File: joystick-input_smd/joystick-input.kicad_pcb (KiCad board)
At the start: 2 copper layers, 53.3 x 35.1 mm, 22 parts, among them J1 Conn_02x18_Odd_Even, J2 Conn_02x14_Odd_Even

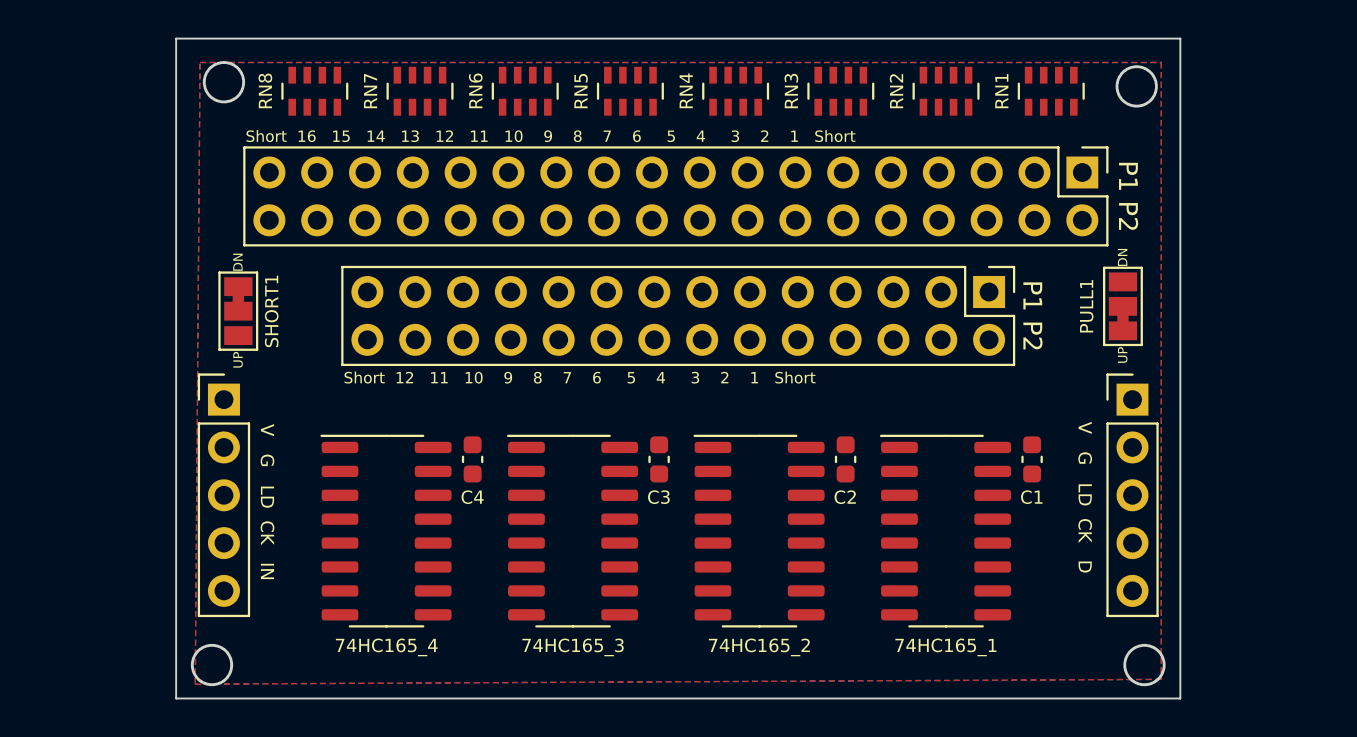
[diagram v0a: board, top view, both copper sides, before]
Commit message: 조이스틱 입력보드 smd 버전 1차 완성
Signed-off-by: Ju, Gyeong-min <jcmh74@gmail.com>
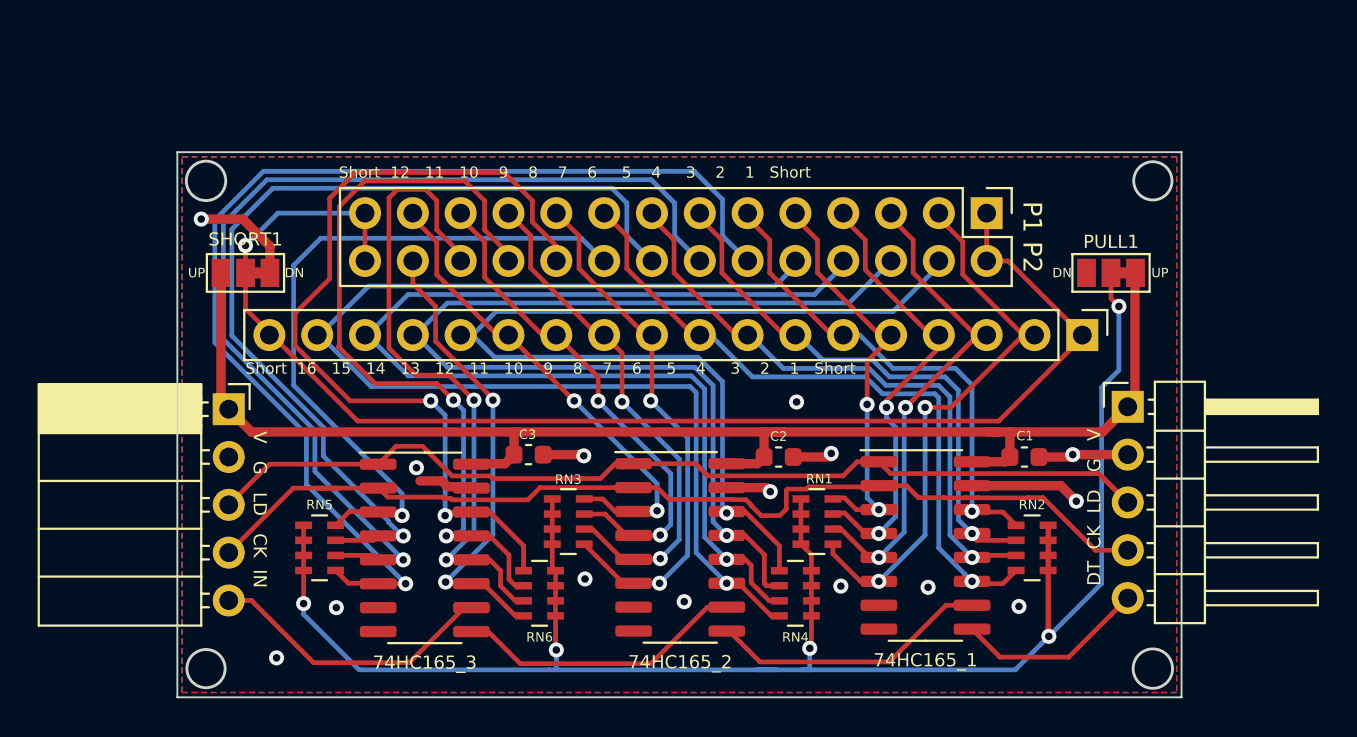
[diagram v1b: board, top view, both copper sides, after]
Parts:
- removed 74HC165_4: 74HC165, Package_SO:SOIC-16_3.9x9.9mm_P1.27mm
- removed C4: C, Capacitor_SMD:C_0603_1608Metric
- removed RN7, RN8: R_Pack04, Resistor_SMD:R_Array_Concave_4x0603
- IN1: footprint Connector_PinHeader_2.54mm:PinHeader_1x05_P2.54mm_Vertical -> Connector_PinSocket_2.54mm:PinSocket_1x05_P2.54mm_Horizontal
- J1: value Conn_02x18_Odd_Even -> Conn_01x18; footprint Connector_PinHeader_2.54mm:PinHeader_2x18_P2.54mm_Vertical -> Connector_PinHeader_2.54mm:PinHeader_1x18_P2.54mm_Vertical
- OUT1: footprint Connector_PinHeader_2.54mm:PinHeader_1x05_P2.54mm_Vertical -> Connector_PinHeader_2.54mm:PinHeader_1x05_P2.54mm_Horizontal
- moved RN5 29.3 mm to (119.4, 89.3), turned to 0 degrees
- moved RN3 27.1 mm to (132.6, 87.9), turned to 0 degrees
- moved RN4 26.9 mm to (144.7, 91.7), turned to 180 degrees
- moved RN6 26.7 mm to (131.1, 91.7), turned to 180 degrees
- moved RN1 26.0 mm to (145.8, 87.9), turned to 0 degrees
- moved RN2 24.7 mm to (157.2, 89.3), turned to 180 degrees
- moved J1 8.64 mm to (159.9, 78.0)
- moved 74HC165_3 7.92 mm to (125.0, 89.3)
- moved C3 6.94 mm to (130.5, 84.3), turned to 0 degrees
- moved 74HC165_2 4.30 mm to (138.5, 89.3)
- moved J2 4.19 mm to (154.8, 71.5)
- moved C2 3.56 mm to (143.8, 84.5), turned to 0 degrees
- moved SHORT1 2.07 mm to (115.4, 74.7), turned to 180 degrees
- moved PULL1 1.89 mm to (161.4, 74.7), turned to 180 degrees
- moved 74HC165_1 1.33 mm to (151.6, 89.2)
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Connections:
- 74HC165_2 pad 11: /C_P1_EX3 -> /C_P2_RIGHT
- 74HC165_2 pad 12: /C_P1_EX2 -> /C_P2_LEFT
- 74HC165_2 pad 13: /C_P1_EX1 -> /C_P2_DOWN
- 74HC165_2 pad 14: /C_P1_HK -> /C_P2_UP
- 74HC165_3 pad 10: /Q7_3 -> /D_IN
- 74HC165_3 pad 11: /C_P2_B -> /C_P2_R
- 74HC165_3 pad 12: /C_P2_A -> /C_P2_L
- 74HC165_3 pad 13: /C_P2_SELECT -> /C_P2_Y
- 74HC165_3 pad 14: /C_P2_START -> /C_P2_X
- 74HC165_3 pad 3: /C_P2_RIGHT -> /C_P2_B
- 74HC165_3 pad 4: /C_P2_LEFT -> /C_P2_A
- 74HC165_3 pad 5: /C_P2_DOWN -> /C_P2_SELECT
- 74HC165_3 pad 6: /C_P2_UP -> /C_P2_START
- J1 pad 10: /C_P2_RIGHT -> /C_P1_X
- J1 pad 11: /C_P1_START -> /C_P1_Y
- J1 pad 12: /C_P2_START -> /C_P1_L
- J1 pad 13: /C_P1_SELECT -> /C_P1_R
- J1 pad 14: /C_P2_SELECT -> /C_P2_UP
- J1 pad 15: /C_P1_A -> /C_P2_DOWN
- J1 pad 16: /C_P2_A -> /C_P2_LEFT
- J1 pad 17: /C_P1_B -> /C_P2_RIGHT
- J1 pad 18: /C_P2_B -> /C_SHORT
- J1 pad 2: /C_SHORT -> /C_P1_UP
- J1 pad 3: /C_P1_UP -> /C_P1_DOWN
- J1 pad 4: /C_P2_UP -> /C_P1_LEFT
- J1 pad 5: /C_P1_DOWN -> /C_P1_RIGHT
- J1 pad 6: /C_P2_DOWN -> /C_P1_START
- J1 pad 7: /C_P1_LEFT -> /C_P1_SELECT
- J1 pad 8: /C_P2_LEFT -> /C_P1_A
- J1 pad 9: /C_P1_RIGHT -> /C_P1_B
- J2 pad 10: /C_P1_EX3 -> /C_P2_RIGHT
- J2 pad 12: /C_P2_UP -> /C_P2_START
- J2 pad 14: /C_P2_DOWN -> /C_P2_SELECT
- J2 pad 16: /C_P2_LEFT -> /C_P2_A
- J2 pad 18: /C_P2_RIGHT -> /C_P2_B
- J2 pad 20: /C_P2_START -> /C_P2_X
- J2 pad 22: /C_P2_SELECT -> /C_P2_Y
- J2 pad 24: /C_P2_A -> /C_P2_L
- J2 pad 26: /C_P2_B -> /C_P2_R
- J2 pad 4: /C_P1_HK -> /C_P2_UP
- J2 pad 6: /C_P1_EX1 -> /C_P2_DOWN
- J2 pad 8: /C_P1_EX2 -> /C_P2_LEFT
- RN1 pad 1: /C_P1_RIGHT -> /PULL
- RN1 pad 2: /C_P1_LEFT -> /PULL
- RN1 pad 3: /C_P1_DOWN -> /PULL
- RN1 pad 4: /C_P1_UP -> /PULL
- RN1 pad 5: /PULL -> /C_P1_UP
- RN1 pad 6: /PULL -> /C_P1_DOWN
- RN1 pad 7: /PULL -> /C_P1_LEFT
- RN1 pad 8: /PULL -> /C_P1_RIGHT
- RN2 pad 1: /C_P1_B -> /PULL
- RN2 pad 2: /C_P1_A -> /PULL
- RN2 pad 3: /C_P1_SELECT -> /PULL
- RN2 pad 4: /C_P1_START -> /PULL
- RN2 pad 5: /PULL -> /C_P1_START
- RN2 pad 6: /PULL -> /C_P1_SELECT
- RN2 pad 7: /PULL -> /C_P1_A
- RN2 pad 8: /PULL -> /C_P1_B
- RN3 pad 1: /C_P1_R -> /PULL
- RN3 pad 2: /C_P1_L -> /PULL
- RN3 pad 3: /C_P1_Y -> /PULL
- RN3 pad 4: /C_P1_X -> /PULL
- RN3 pad 5: /PULL -> /C_P1_X
- RN3 pad 6: /PULL -> /C_P1_Y
- RN3 pad 7: /PULL -> /C_P1_L
- RN3 pad 8: /PULL -> /C_P1_R
- RN4 pad 1: /C_P1_EX3 -> /PULL
- RN4 pad 2: /C_P1_EX2 -> /PULL
- RN4 pad 3: /C_P1_EX1 -> /PULL
- RN4 pad 4: /C_P1_HK -> /PULL
- RN4 pad 5: /PULL -> /C_P2_UP
- RN4 pad 6: /PULL -> /C_P2_DOWN
- RN4 pad 7: /PULL -> /C_P2_LEFT
- RN4 pad 8: /PULL -> /C_P2_RIGHT
- RN5 pad 1: /C_P2_RIGHT -> /PULL
- RN5 pad 2: /C_P2_LEFT -> /PULL
- RN5 pad 3: /C_P2_DOWN -> /PULL
- RN5 pad 4: /C_P2_UP -> /PULL
- RN5 pad 5: /PULL -> /C_P2_START
- RN5 pad 6: /PULL -> /C_P2_SELECT
- RN5 pad 7: /PULL -> /C_P2_A
- RN5 pad 8: /PULL -> /C_P2_B
- RN6 pad 1: /C_P2_B -> /PULL
- RN6 pad 2: /C_P2_A -> /PULL
- RN6 pad 3: /C_P2_SELECT -> /PULL
- RN6 pad 4: /C_P2_START -> /PULL
- RN6 pad 5: /PULL -> /C_P2_X
- RN6 pad 6: /PULL -> /C_P2_Y
- RN6 pad 7: /PULL -> /C_P2_L
- RN6 pad 8: /PULL -> /C_P2_R
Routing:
- net /PULL: track 0.00 -> 99.9 mm, vias 0 -> 5
- net VCC: track 0.00 -> 75.3 mm
- net /C_SHORT: track 0.00 -> 72.1 mm, vias 0 -> 1
- net /C_P2_RIGHT: track 0.00 -> 62.4 mm, vias 0 -> 1
- net /C_P2_START: track 0.00 -> 60.0 mm, vias 0 -> 1
- net /C_P2_LEFT: track 0.00 -> 59.7 mm, vias 0 -> 1
- net /C_P2_DOWN: track 0.00 -> 56.9 mm, vias 0 -> 1
- net /CLK: track 0.00 -> 55.1 mm
- net /C_P2_SELECT: track 0.00 -> 54.6 mm, vias 0 -> 1
- net /LOAD: track 0.00 -> 53.2 mm
- net /C_P2_UP: track 0.00 -> 52.6 mm, vias 0 -> 1
- net /C_P2_A: track 0.00 -> 49.6 mm, vias 0 -> 1
- net /C_P2_X: track 0.00 -> 45.4 mm, vias 0 -> 2
- net /C_P2_Y: track 0.00 -> 41.3 mm, vias 0 -> 2
- net /C_P2_B: track 0.00 -> 37.2 mm, vias 0 -> 1
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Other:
- board size 53.3 x 35.1 mm -> 53.3 x 29 mm
- board text added: "DT CK LD G V"
- board text removed: "V G LD CK D"
